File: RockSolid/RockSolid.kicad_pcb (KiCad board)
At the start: 2 copper layers, 25 parts, among them J1 Conn_01x06, Q1 IRF510, U1 L78L05_TO92, U2 74HC04, Y1 10 Mhz

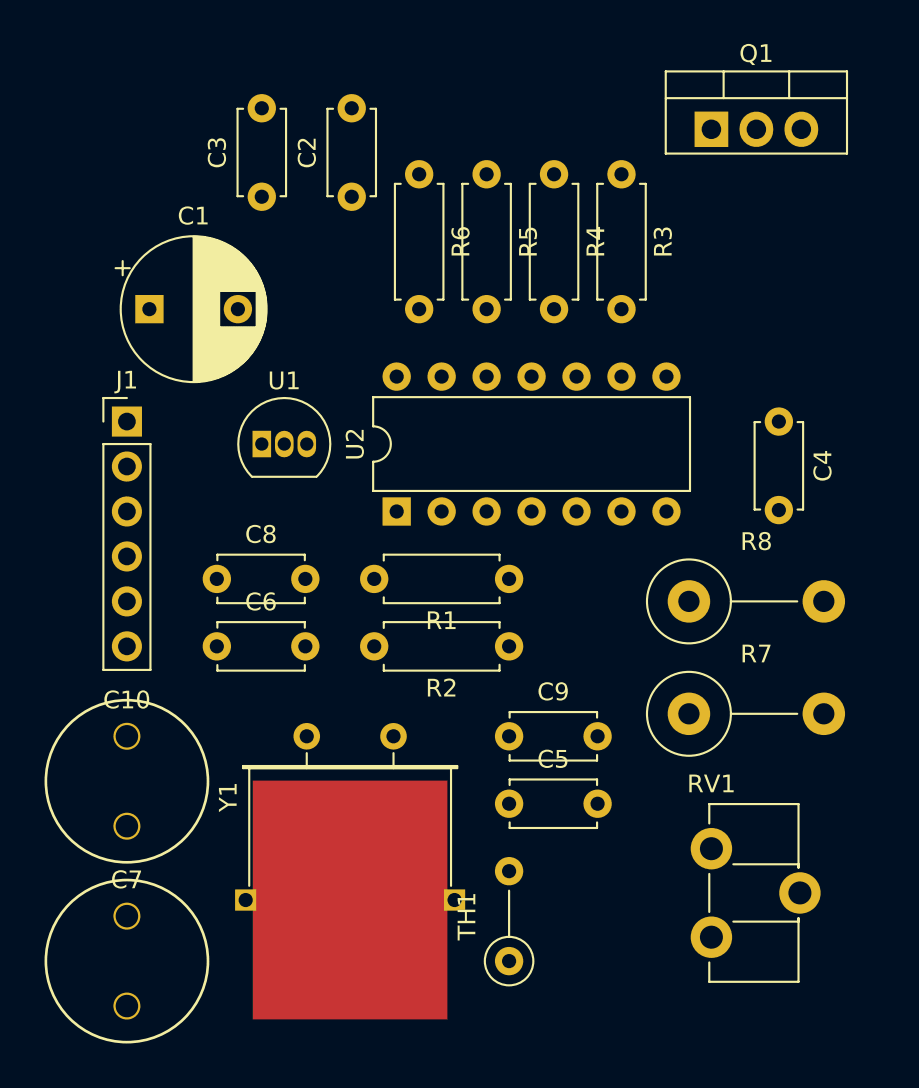
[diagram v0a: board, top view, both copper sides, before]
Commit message: Initial version before changes.
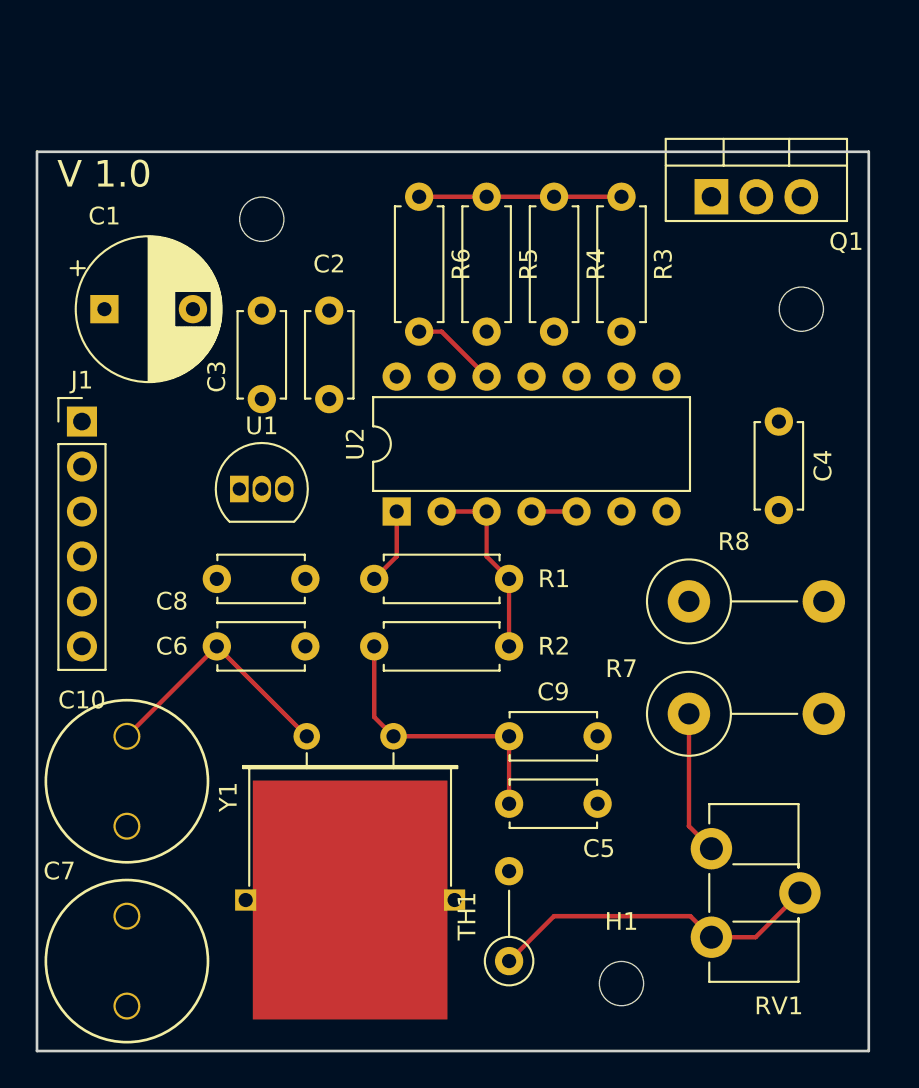
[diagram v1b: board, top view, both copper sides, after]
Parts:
- added H1: MountingHole, MountingHole:MountingHole_2.5mm, F.Cu at (102.9, 92.7)
- added H2: MountingHole, MountingHole:MountingHole_2.5mm, F.Cu at (113.0, 54.6)
- added H3: MountingHole, MountingHole:MountingHole_2.5mm, F.Cu at (82.5, 49.5)
- moved C2 11.5 mm to (86.4, 59.7)
- moved C3 11.4 mm to (82.5, 59.7)
- moved Q1 3.81 mm to (108.0, 48.3)
- moved U1 2.84 mm to (81.3, 64.8)
- moved C1 2.54 mm to (73.7, 54.6)
- moved J1 2.54 mm to (72.4, 61.0)
- moved R3 1.27 mm to (102.9, 48.3)
- moved R4 1.27 mm to (99.1, 48.3)
- moved R5 1.27 mm to (95.2, 48.3)
- moved R6 1.27 mm to (91.4, 48.3)
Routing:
- net Net-(Q1-Pad1): track 0.00 -> 19.0 mm
- net Net-(C10-Pad1): track 0.00 -> 18.7 mm
- net Net-(C5-Pad1): track 0.00 -> 15.9 mm
- net Net-(J1-Pad4): track 0.00 -> 11.4 mm
- net Net-(R1-Pad1): track 0.00 -> 10.7 mm
- net Net-(J1-Pad6): track 0.00 -> 8.15 mm
- net Net-(R6-Pad2): track 0.00 -> 4.86 mm
- net Net-(J1-Pad3): track 0.00 -> 2.54 mm
- added copper zone on B.Cu, net GND
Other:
- board outline added: 47 x 50.8 mm
- board text added: "Rock Solid OCXO (c) 2021 Will Cooke smalltimeelectronics.com"
- board text added: "V 1.0"

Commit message: Version 1.0RC1 complete.
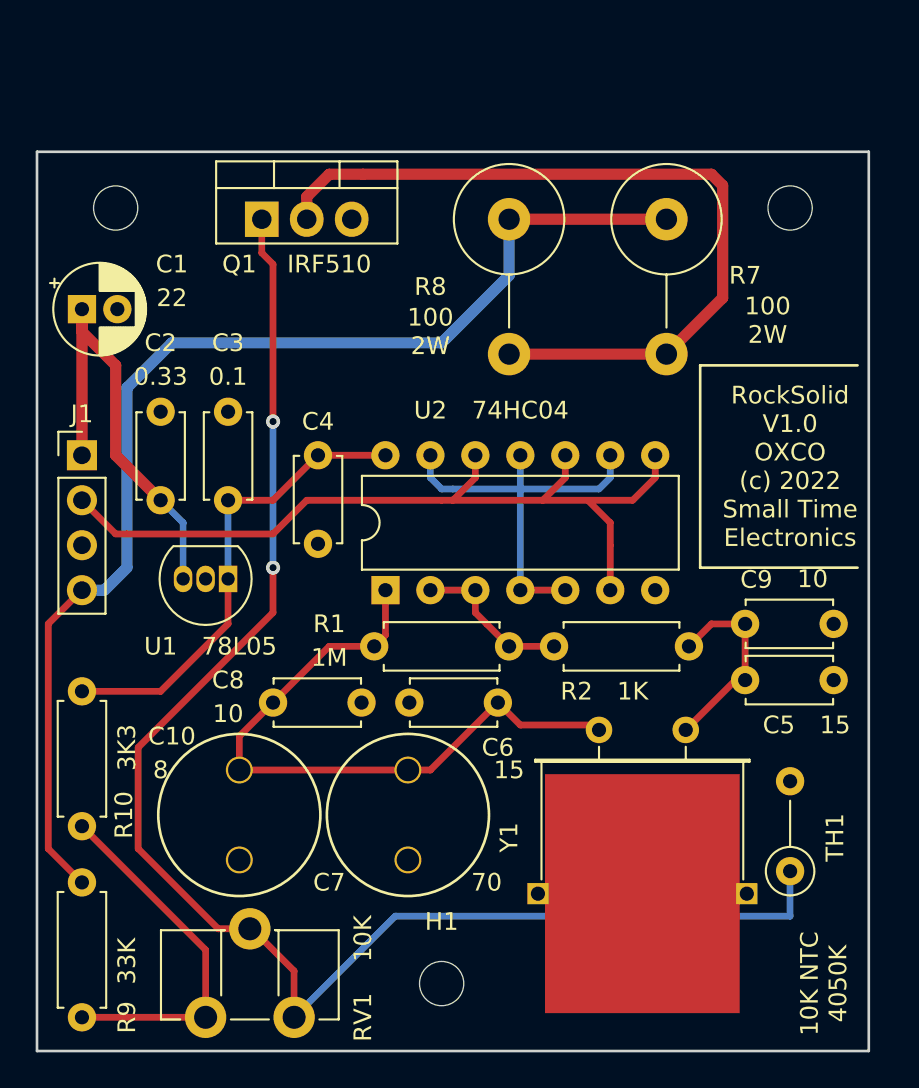
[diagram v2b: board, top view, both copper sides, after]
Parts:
- removed R3, R4, R5, R6: 180, Resistor_THT:R_Axial_DIN0207_L6.3mm_D2.5mm_P7.62mm_Horizontal
- added R10: 3K3, Resistor_THT:R_Axial_DIN0207_L6.3mm_D2.5mm_P7.62mm_Horizontal, F.Cu at (72.4, 76.2)
- added R9: 33K, Resistor_THT:R_Axial_DIN0207_L6.3mm_D2.5mm_P7.62mm_Horizontal, F.Cu at (72.4, 87.0)
- C1: footprint Capacitor_THT:CP_Radial_D8.0mm_P5.00mm -> Capacitor_THT:CP_Radial_D5.0mm_P2.00mm
- J1: value Conn_01x06 -> Conn_01x04; footprint Connector_PinHeader_2.54mm:PinHeader_1x06_P2.54mm_Vertical -> Connector_PinHeader_2.54mm:PinHeader_1x04_P2.54mm_Vertical
- R7, R8: footprint Resistor_THT:R_Axial_DIN0414_L11.9mm_D4.5mm_P7.62mm_Vertical -> Resistor_THT:R_Axial_DIN0617_L17.0mm_D6.0mm_P7.62mm_Vertical
- RV1: value 50K -> 10K
- moved RV1 30.1 mm to (79.4, 94.6), turned to 90 degrees
- moved R7 28.0 mm to (105.4, 49.5), turned to 270 degrees
- moved C4 26.1 mm to (85.7, 62.9)
- moved Q1 25.4 mm to (82.5, 49.5)
- moved R8 23.9 mm to (96.5, 49.5), turned to 270 degrees
- moved C7 17.9 mm to (90.8, 80.6)
- moved TH1 16.7 mm to (112.4, 86.4)
- moved Y1 16.5 mm to (101.6, 78.4)
- moved C6 16.2 mm to (95.9, 76.8), turned to 180 degrees
- moved C5 15.1 mm to (109.9, 75.6)
- moved C9 14.8 mm to (109.9, 72.4)
- moved C2 11.1 mm to (76.8, 65.4)
- moved H1 10.2 mm to (92.7, 92.7)
- moved H3 8.28 mm to (74.3, 48.9)
- moved C8 7.67 mm to (83.2, 76.8)
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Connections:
- J1 pad 2: GND -> Net-(J1-Pad2)
- J1 pad 3: Net-(J1-Pad3) -> GND
- R7 pad 1: Net-(J1-Pad6) -> Net-(J1-Pad4)
- R8 pad 1: Net-(J1-Pad6) -> Net-(J1-Pad4)
- RV1 pad 1: Net-(J1-Pad6) -> Net-(R10-Pad2)
- U2 pad 10: Net-(R5-Pad2) -> Net-(J1-Pad2)
- U2 pad 11: Net-(J1-Pad3) -> Net-(U2-Pad11)
- U2 pad 12: Net-(R6-Pad2) -> Net-(J1-Pad2)
- U2 pad 13: Net-(J1-Pad3) -> Net-(U2-Pad11)
- U2 pad 4: Net-(J1-Pad3) -> Net-(U2-Pad11)
- U2 pad 5: Net-(J1-Pad3) -> Net-(U2-Pad11)
- U2 pad 6: Net-(R3-Pad2) -> Net-(J1-Pad2)
- U2 pad 8: Net-(R4-Pad2) -> Net-(J1-Pad2)
- U2 pad 9: Net-(J1-Pad3) -> Net-(U2-Pad11)
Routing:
- net Net-(Q1-Pad1): track 19.0 -> 86.2 mm, vias 0 -> 2
- net Net-(J1-Pad4): track 11.4 -> 67.6 mm
- net Net-(J1-Pad2): track 0.00 -> 47.5 mm
- net Net-(Q1-Pad2): track 0.00 -> 45.3 mm
- net VCC: track 0.00 -> 26.8 mm
- net Net-(C1-Pad1): track 0.00 -> 25.9 mm
- net Net-(U2-Pad11): track 0.00 -> 23.4 mm
- net Net-(R10-Pad2): track 0.00 -> 20.7 mm
- net Net-(C10-Pad1): track 18.7 -> 38.1 mm
- net Net-(Y1-Pad3): track 0.00 -> 17.5 mm
- net Net-(J1-Pad6): track 8.15 -> 0.00 mm
- net Net-(R6-Pad2): track 4.86 -> 0.00 mm
- net Net-(C5-Pad1): track 15.9 -> 11.4 mm
- net Net-(J1-Pad3): track 2.54 -> 0.00 mm
- net Net-(R1-Pad1): track 10.7 -> 9.04 mm
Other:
- board text added: "0.1"
- board text added: "0.33"
- board text added: "10"
- board text added: "100 2W"
- board text added: "10K"
- board text added: "10K NTC 4050K"
- board text added: "15"
- board text added: "1K"
- board text added: "1M"
- board text added: "22"
- board text added: "33K"
- board text added: "3K3"
- board text added: "70"
- board text added: "74HC04"
- board text added: "78L05"
- board text added: "8"
- board text added: "IRF510"
- board text added: "RockSolid V1.0 OXCO (c) 2022 Small Time Electronics"
- board text removed: "V 1.0"
